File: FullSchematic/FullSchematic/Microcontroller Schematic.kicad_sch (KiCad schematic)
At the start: 30 parts, among them J1 USB_B_Micro, J3 Conn_01x24_Socket, J4 Conn_01x24_Socket, U2 FT231XS, U3 24LC64

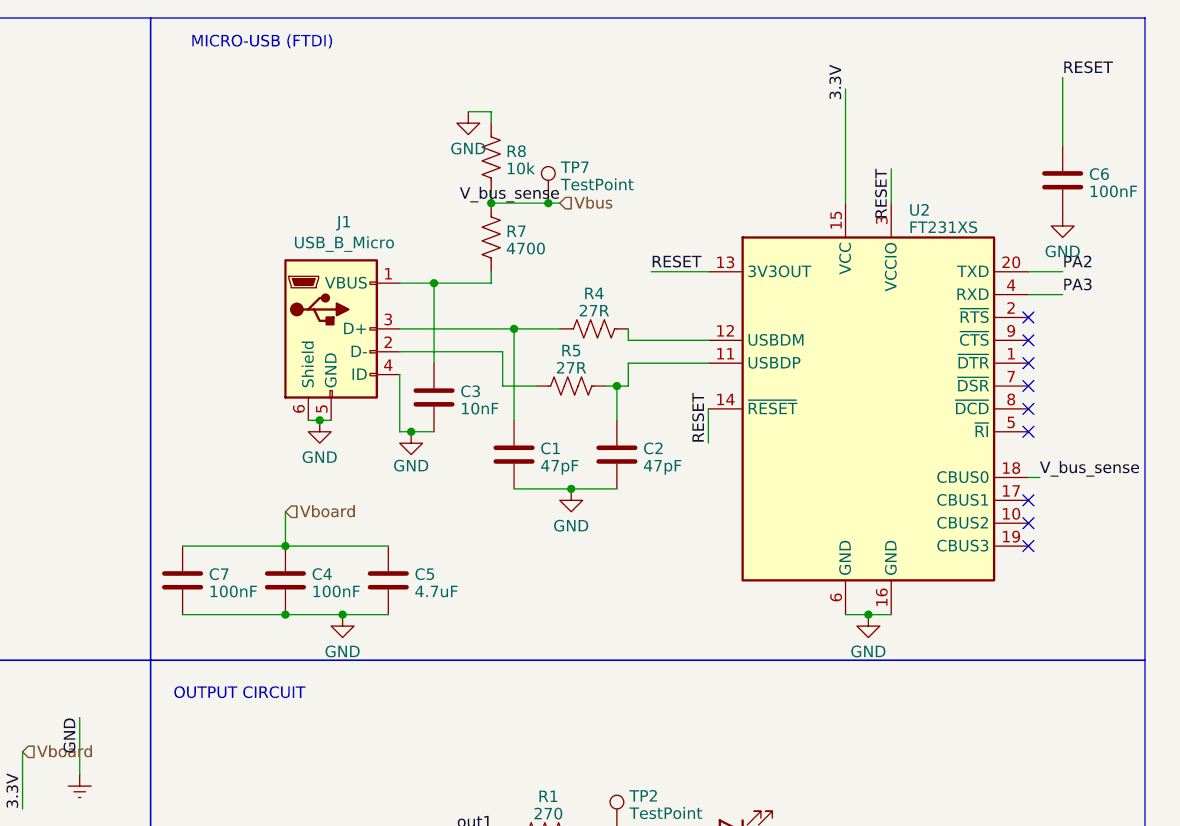
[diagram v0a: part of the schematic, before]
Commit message: Corrected errors
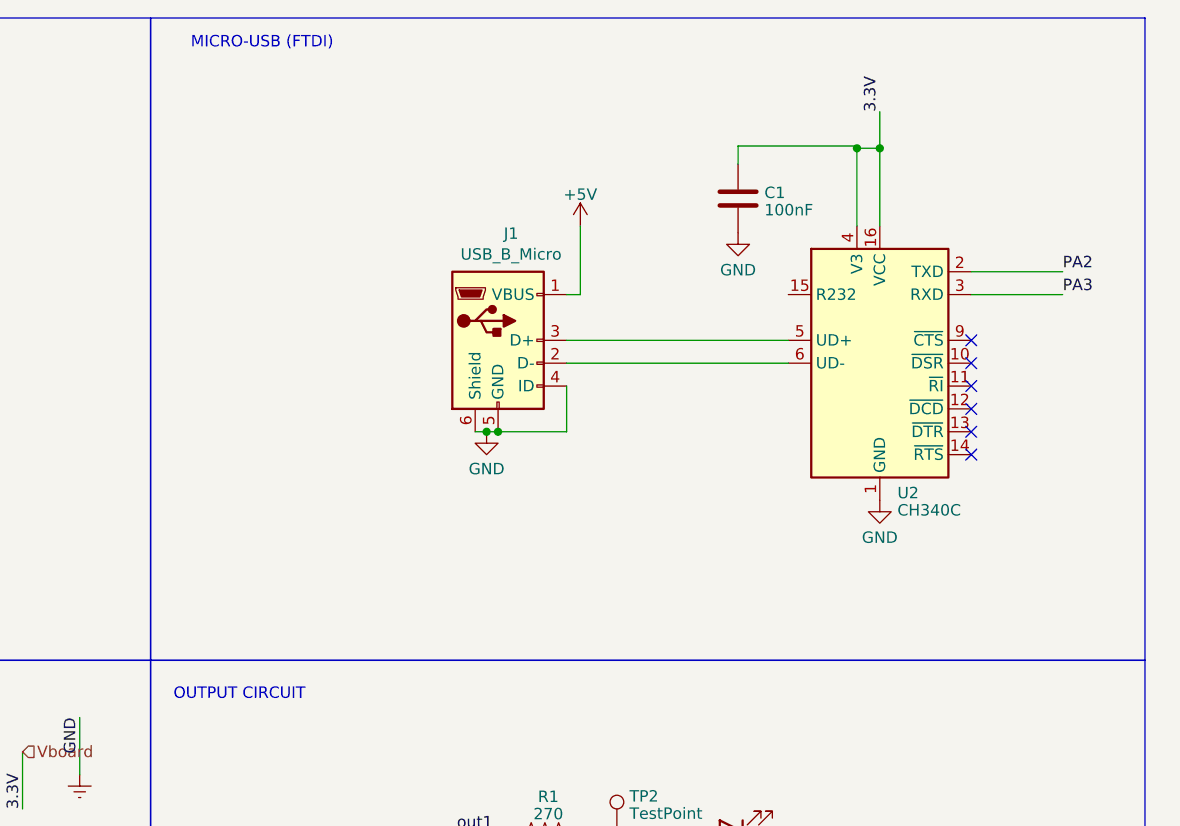
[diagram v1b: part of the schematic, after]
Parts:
- removed C2: 47pF, symbol Device:C
- removed C3: 10nF, symbol Device:C
- removed C4, C6, C7: 100nF, symbol Device:C
- removed C5: 4.7uF, symbol Device:C
- removed R4, R5: 27R, symbol Device:R_US
- removed R7: 4700, symbol Device:R_US
- removed R8: 10k, symbol Device:R_US
- removed TP7: TestPoint, symbol Connector:TestPoint
- removed U2: FT231XS, Package_SO:SSOP-20_3.9x8.7mm_P0.635mm, symbol Interface_USB:FT231XS
- added U2: CH340C, Package_SO:SOIC-16_3.9x9.9mm_P1.27mm, symbol Interface_USB:CH340C
- C1: value 47pF -> 100nF; JLCPCB Part # C105622 -> C24497; Price $0.0447 -> 0.08; Price ( 1 board) 0.0894 -> 0.32; Price (5 boards) 0.447 -> 1.6
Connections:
- net Earth: now also U2.1 (GND)
- net PA2: now also U2.2 (TXD)
- net PA3: now also U2.3 (RXD)
- net Vboard: now also C1.1, U2.16 (VCC), U2.4 (V3)
- net +5V: now reaches J1.1 (VBUS)
- net at J1.2 (D-): now also U2.6 (UD-)
- net at J1.3 (D+): now also U2.5 (UD+); no longer C1.1
- no-connect marks 42 -> 39
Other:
- moved on the sheet: J1
